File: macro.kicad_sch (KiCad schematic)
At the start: 28 parts, among them SW1 SW_Push, U1 ATmega32U4-A, Y1 16MHz

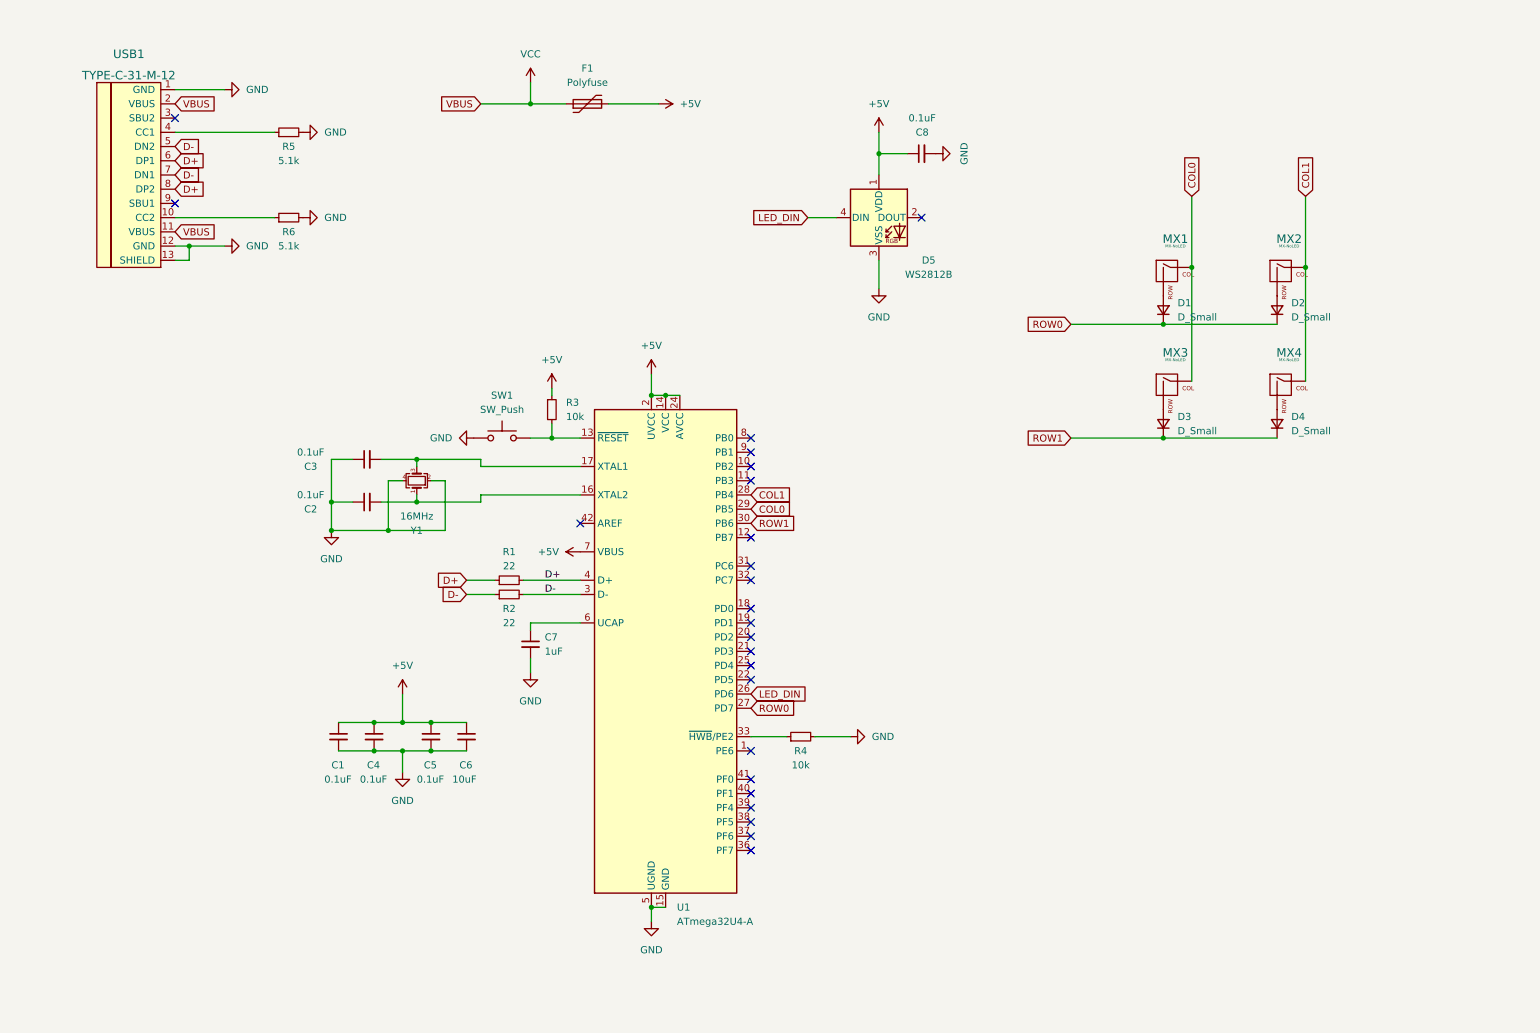
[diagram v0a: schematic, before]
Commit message: New design
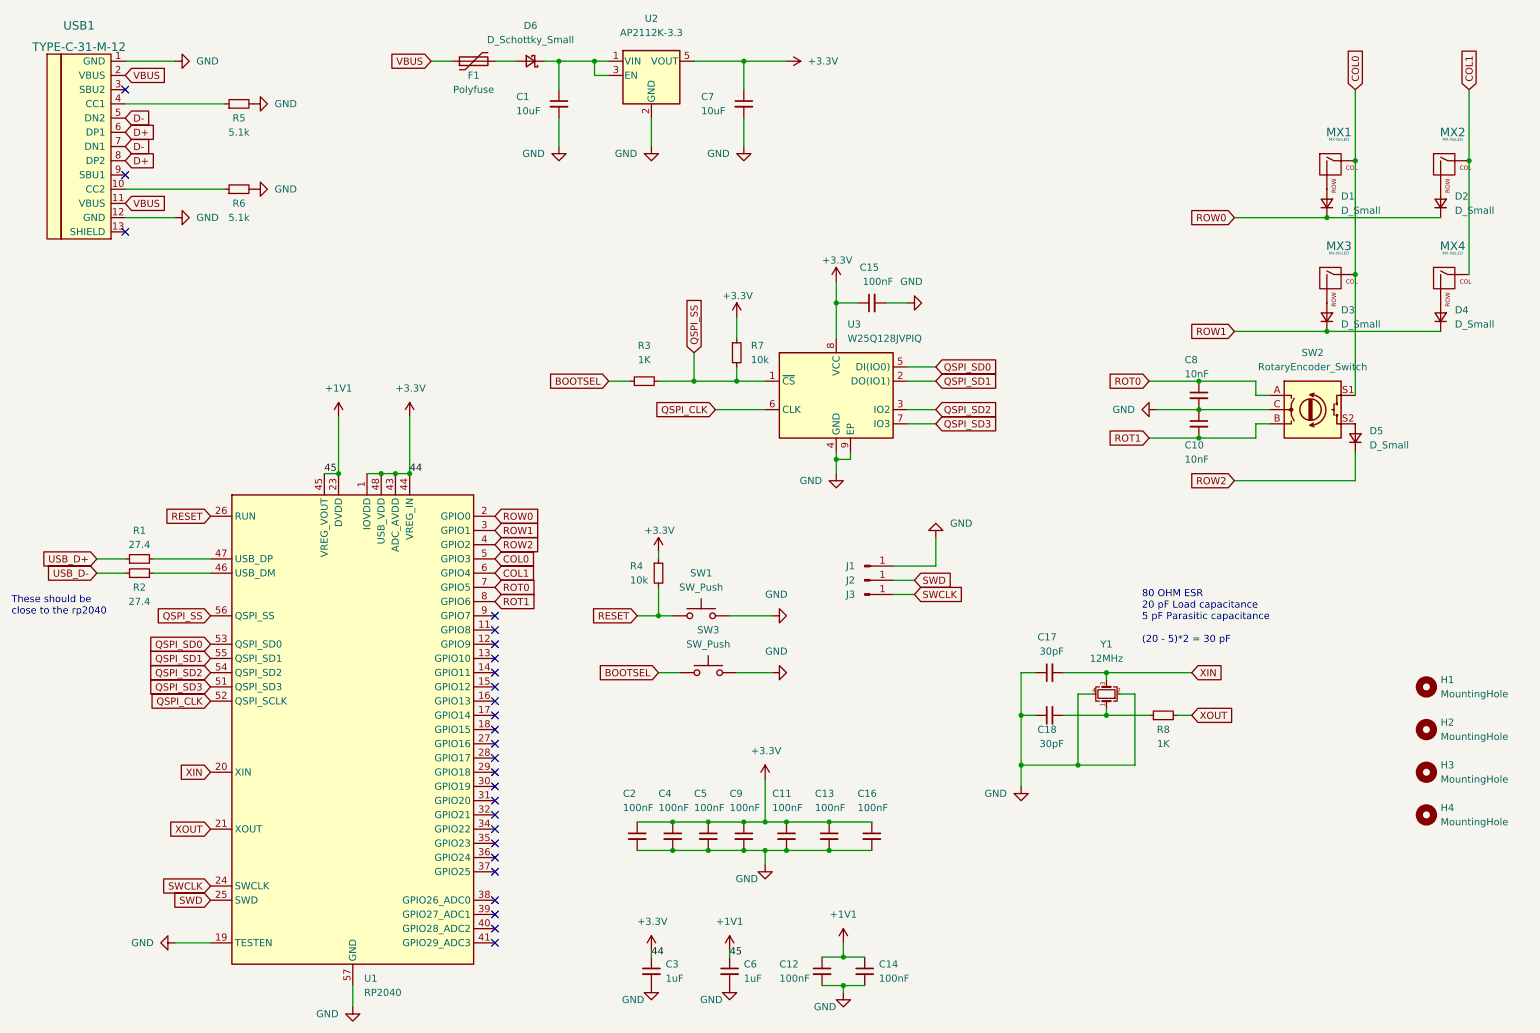
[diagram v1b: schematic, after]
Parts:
- removed D5: WS2812B, LED_SMD:LED_WS2812B_PLCC4_5.0x5.0mm_P3.2mm, symbol LED:WS2812B
- removed U1: ATmega32U4-A, Package_QFP:TQFP-44_10x10mm_P0.8mm, symbol MCU_Microchip_ATmega:ATmega32U4-A
- added C10: 10nF, Capacitor_SMD:C_0402_1005Metric, symbol Device:C_Small
- added C11, C12, C13, C14, C15, C16, C9: 100nF, Capacitor_SMD:C_0402_1005Metric, symbol Device:C_Small
- added C17, C18: 30pF, Capacitor_SMD:C_0402_1005Metric, symbol Device:C_Small
- added D5: D_Small, Diode_SMD:D_SOD-323, symbol Device:D_Small
- added D6: D_Schottky_Small, Diode_SMD:D_SOD-323, symbol Device:D_Schottky_Small
- added H1, H2, H3, H4: MountingHole, MountingHole:MountingHole_2.2mm_M2, symbol Mechanical:MountingHole
- added J1, J2, J3: Conn_01x01_Male, TestPoint:TestPoint_Pad_2.0x2.0mm, symbol Connector:Conn_01x01_Male
- added R7: 10k, Resistor_SMD:R_0402_1005Metric, symbol Device:R_Small
- added R8: 1K, Resistor_SMD:R_0402_1005Metric, symbol Device:R_Small
- added SW2: RotaryEncoder_Switch, Rotary_Encoder:RotaryEncoder_Alps_EC11E-Switch_Vertical_H20mm_CircularMountingHoles, symbol Device:RotaryEncoder_Switch
- added SW3: SW_Push, Button_Switch_SMD:SW_Push_1P1T_NO_CK_KMR2, symbol Switch:SW_Push
- added U1: RP2040, Package_DFN_QFN:QFN-56-1EP_7x7mm_P0.4mm_EP3.2x3.2mm, symbol rp2040:RP2040
- added U2: AP2112K-3.3, Package_TO_SOT_SMD:SOT-23-5, symbol Regulator_Linear:AP2112K-3.3
- added U3: W25Q128JVPIQ, Package_SON:WSON-8-1EP_6x5mm_P1.27mm_EP3.4x4.3mm, symbol Memory_Flash:W25Q32JVZP
- C1: value 0.1uF -> 10uF; footprint Capacitor_SMD:C_0805_2012Metric_Pad1.18x1.45mm_HandSolder -> Capacitor_SMD:C_0402_1005Metric
- C2, C4, C5: value 0.1uF -> 100nF; footprint Capacitor_SMD:C_0805_2012Metric_Pad1.18x1.45mm_HandSolder -> Capacitor_SMD:C_0402_1005Metric
- C3: value 0.1uF -> 1uF; footprint Capacitor_SMD:C_0805_2012Metric_Pad1.18x1.45mm_HandSolder -> Capacitor_SMD:C_0402_1005Metric
- C6: value 10uF -> 1uF; footprint Capacitor_SMD:C_0805_2012Metric_Pad1.18x1.45mm_HandSolder -> Capacitor_SMD:C_0402_1005Metric
- C7: value 1uF -> 10uF; footprint Capacitor_SMD:C_0805_2012Metric_Pad1.18x1.45mm_HandSolder -> Capacitor_SMD:C_0402_1005Metric
- C8: value 0.1uF -> 10nF; footprint Capacitor_SMD:C_0805_2012Metric_Pad1.18x1.45mm_HandSolder -> Capacitor_SMD:C_0402_1005Metric
- D1, D2, D3, D4: footprint Diode_SMD:D_SOD-123 -> Diode_SMD:D_SOD-323
- F1: footprint Fuse:Fuse_1206_3216Metric -> Fuse:Fuse_0402_1005Metric
- R1, R2: value 22 -> 27.4; footprint Resistor_SMD:R_0805_2012Metric -> Resistor_SMD:R_0402_1005Metric
- R3: value 10k -> 1K; footprint Resistor_SMD:R_0805_2012Metric -> Resistor_SMD:R_0402_1005Metric
- R4, R5, R6: footprint Resistor_SMD:R_0805_2012Metric -> Resistor_SMD:R_0402_1005Metric
- SW1: footprint random-keyboard-parts:SKQG-1155865 -> Button_Switch_SMD:SW_Push_1P1T_NO_CK_KMR2
- Y1: value 16MHz -> 12MHz
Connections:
- net COL0: now also SW2.S1, U1.5 (GPIO3)
- net COL1: now also U1.6 (GPIO4)
- net D+: no longer R1.1, R1.2
- net D-: no longer R2.1, R2.2
- net GND: now also C2.2, C3.2, SW1.2, C10.1, C11.2, C12.2, C13.2, C14.2, C15.2, C16.2, C17.1, C18.1, C9.2, J1.1 (Pin_1), SW2.C, SW3.2, U1.19 (TESTEN), U1.57 (GND), U2.2 (GND), U3.4 (GND), U3.9 (EP); no longer C2.1, C3.1, R4.2, SW1.1, USB1.13 (SHIELD)
- net ROW0: now also U1.2 (GPIO0)
- net ROW1: now also U1.3 (GPIO1)
- net at Y1.1: now also C18.2, R8.1; no longer C2.2
- net XIN: now reaches Y1.3
- net XIN: now also C17.2, U1.20 (XIN); no longer C3.2
- net QSPI_SS: now reaches R3.2
- net QSPI_SS: now also R7.2, U1.56 (QSPI_SS), U3.1 (~{CS}); no longer SW1.2
- net +3.3V: now reaches C7.1
- net +3.3V: now also C2.1, C3.1, C4.1, C5.1, R4.1, C11.1, C13.1, C15.1, C16.1, C9.1, R7.1, U1.1 (IOVDD), U1.10 (IOVDD), U1.22 (IOVDD), U1.33 (IOVDD), U1.42 (IOVDD), U1.43 (ADC_AVDD), U1.44 (VREG_IN), U1.48 (USB_VDD), U1.49 (IOVDD), U2.5 (VOUT), U3.8 (VCC)
- removed net +5V: C1.1, C4.1, C5.1, C6.1, C8.1, F1.2, R3.1
- net VCC renamed VBUS
- new net: C1.1, D6.1 (K), U2.1 (VIN), U2.3 (EN)
- new net: D6.2 (A), F1.2
- new net: R1.2, U1.47 (USB_DP)
- new net: R2.2, U1.46 (USB_DM)
- new net: D5.2 (A), SW2.S2
- new net +1V1: C12.1, C14.1, C6.1, U1.23 (DVDD), U1.45 (VREG_VOUT), U1.50 (DVDD)
- new net BOOTSEL: R3.1, SW3.1
- new net QSPI_CLK: U1.52 (QSPI_SCLK), U3.6 (CLK)
- new net QSPI_SD0: U1.53 (QSPI_SD0), U3.5 (DI(IO0))
- new net QSPI_SD1: U1.55 (QSPI_SD1), U3.2 (DO(IO1))
- new net QSPI_SD2: U1.54 (QSPI_SD2), U3.3 (IO2)
- new net QSPI_SD3: U1.51 (QSPI_SD3), U3.7 (IO3)
- new net RESET: R4.2, SW1.1, U1.26 (RUN)
- new net ROT0: C8.1, SW2.A, U1.7 (GPIO5)
- new net ROT1: C10.2, SW2.B, U1.8 (GPIO6)
- new net ROW2: D5.1 (K), U1.4 (GPIO2)
- new net SWCLK: J3.1 (Pin_1), U1.24 (SWCLK)
- new net SWD: J2.1 (Pin_1), U1.25 (SWD)
- new net USB_D+: R1.1
- new net USB_D-: R2.1
- new net XOUT: R8.2, U1.21 (XOUT)
- no-connect marks 24 -> 26
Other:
- note added: "80 OHM ESR 20 pF Load capacitance 5 pF Parasitic capacitance (20 - 5)*2 = 30 pF"
- note added: "These should be close to the rp2040"
- moved on the sheet: D1, D2, D3, D4, MX1, MX2, MX3, MX4, R5, R6, USB1
